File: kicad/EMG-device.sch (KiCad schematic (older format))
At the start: 53 parts

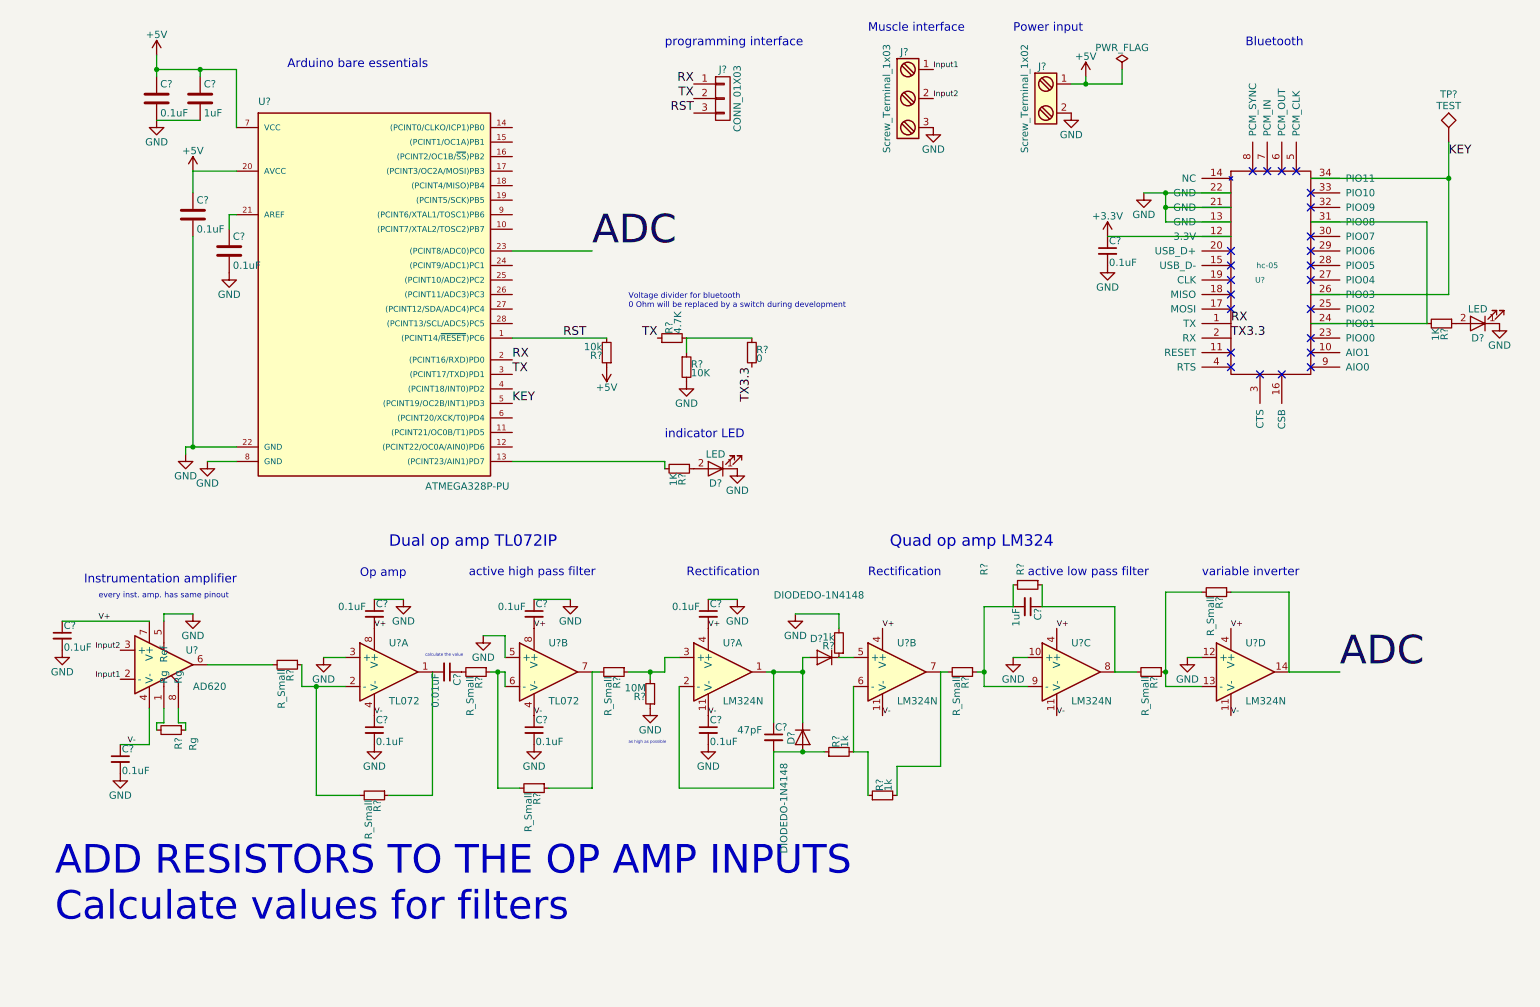
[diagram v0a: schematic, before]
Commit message: schematics done
schematics 1.0 done
BOM updated, but not ready
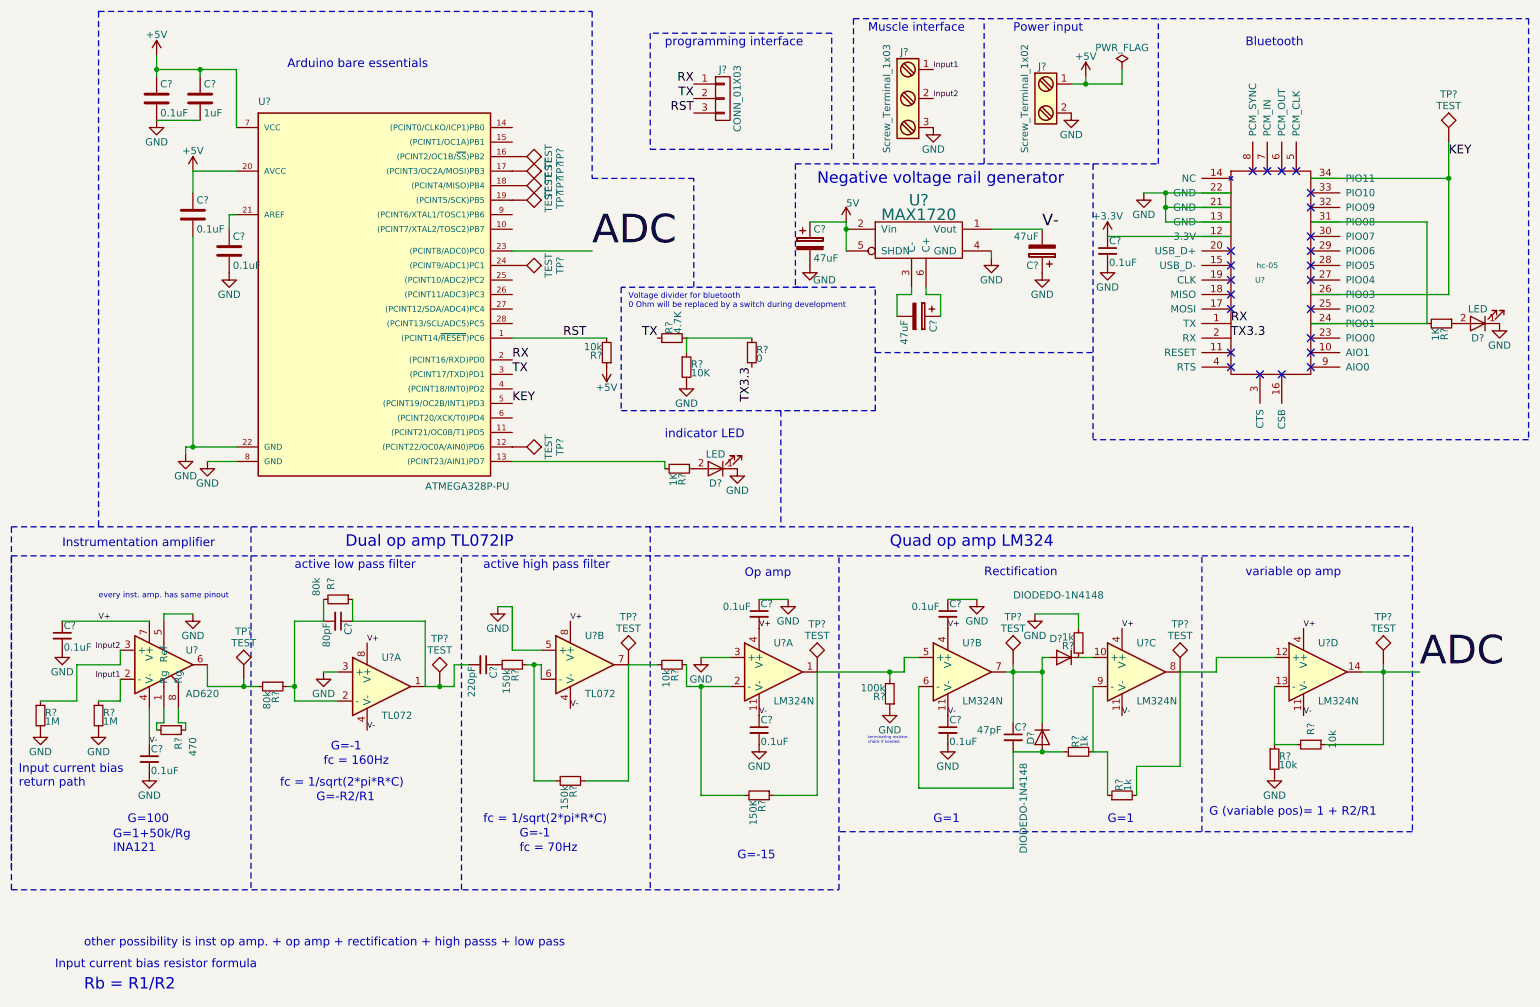
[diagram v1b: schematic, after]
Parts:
- removed C? (x2): 0.1uF, symbol C_Small
- removed R? (x3): R_Small, symbol R_Small
- added C? (x3): 47uF, symbol CP
- added R? (x2): 1M, symbol R_Small
- added R? (x2): 10k, symbol R_Small
- added TP? (x13): TEST, symbol TEST
- added U?: MAX1720, symbol MAX1720
- C?: value 0.01uF -> 220pF
- C?: value 1uF -> 80pF
- R?: value Rg -> 470
- R?: value R_Small -> 10k
- R?: value R_Small -> 150K
- R? (x2): value R_Small -> 150k
- R?: value 10M -> 100k
- R?: value R_Small -> 80k
- R?: value R? -> 80k
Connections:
- net ADC: now also R?.1, TP?.1
- net GND: now also U?.3 (+), C?.1, C?.2, R?.2, R?.2, R?.2, U?.4 (GND); no longer U?.10 (+), U?.12 (+)
- net Input1: now also R?.1
- net Input2: now also R?.1
- net V-: now also C?.2, U?.1 (Vout)
- net at U?.12 ((PCINT22/OC0A/AIN0)PD6): now also TP?.1
- net at U?.16 ((PCINT2/OC1B/~SS~)PB2): now also TP?.1
- net at U?.17 ((PCINT3/OC2A/MOSI)PB3): now also TP?.1
- net at U?.18 ((PCINT4/MISO)PB4): now also TP?.1
- net at U?.19 ((PCINT5/SCK)PB5): now also TP?.1
- net at U?.24 ((PCINT9/ADC1)PC1): now also TP?.1
- net at U?.6: now also R?.2, TP?.1; no longer R?.2
- net at C?.2, U?.1: now also C?.1, R?.1, TP?.1; no longer R?.1
- net at R?.1, R?.2: now also U?.2 (-); no longer U?.2 (-)
- net at R?.1, U?.7: now also R?.2, TP?.1
- net at C?.1, D?.A, D?.C: now also U?.7, TP?.1; no longer U?.1
- net at C?.2, D?.A, R?.1: now also U?.6 (-); no longer U?.2 (-)
- net at R?.2: now also R?.1, U?.1, U?.5 (+), TP?.1; no longer U?.3 (+)
- net at D?.C, R?.1: now also U?.10 (+); no longer U?.5 (+)
- net at R?.1, R?.2: now also U?.9 (-); no longer U?.6 (-)
- net at C?.2, R?.1, R?.2: now also U?.2 (-); no longer U?.9 (-)
- net at U?.13 (-): now also R?.1, R?.2
- new net: R?.2, TP?.1, U?.12 (+), U?.8
- new net: C?.2, U?.3 (C-)
- new net: C?.1, U?.6 (C+)
- new net 5V: C?.1, U?.2 (Vin), U?.5 (SHDN)
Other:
- note added: "G (variable pos)= 1 + R2/R1\n"
- note added: "G=-1"
- note added: "G=-15"
- note added: "G=-1\n"
- note added: "G=-R2/R1"
- note added: "G=1"
- note added: "G=1+50k/Rg\nINA121"
- note added: "G=100"
- note added: "Input current bias \nreturn path"
- note added: "Input current bias resistor formula"
- note added: "Negative voltage rail generator"
- note added: "Rb = R1/R2"
- note added: "fc = 1/sqrt(2*pi*R*C)"
- note added: "fc = 160Hz"
- note added: "fc = 70Hz"
- note added: "other possibility is inst op amp. + op amp + rectification + high passs + low pass"
- note added: "terminating resistor,\ncheck if needed\n"
- note added: "variable op amp\n"
- note removed: "ADD RESISTORS TO THE OP AMP INPUTS\nCalculate values for filters\n\n"
- note removed: "as high as possible\n"
- note removed: "calculate the value\n"
- note removed: "variable inverter\n"
- moved on the sheet: C?, D?, R?, U?A, U?B, U?C, U?D
